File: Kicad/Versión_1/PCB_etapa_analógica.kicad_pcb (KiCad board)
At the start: 2 copper layers, 83 x 63 mm, 44 parts, among them J1 Conn_01x01_Pin, J12 Conn_01x01_Pin, J13 Conn_01x01_Pin, J14 Conn_01x01_Pin, J15 Conn_01x01_Pin, J2 Conn_01x01_Pin, J3 Conn_01x01_Pin, J4 Conn_01x01_Pin, J5 Conn_01x01_Pin, J6 Conn_01x01_Pin, J7 Conn_01x01_Pin, U1 AD620, U2 TL084, U4 TL084, U5 TL082

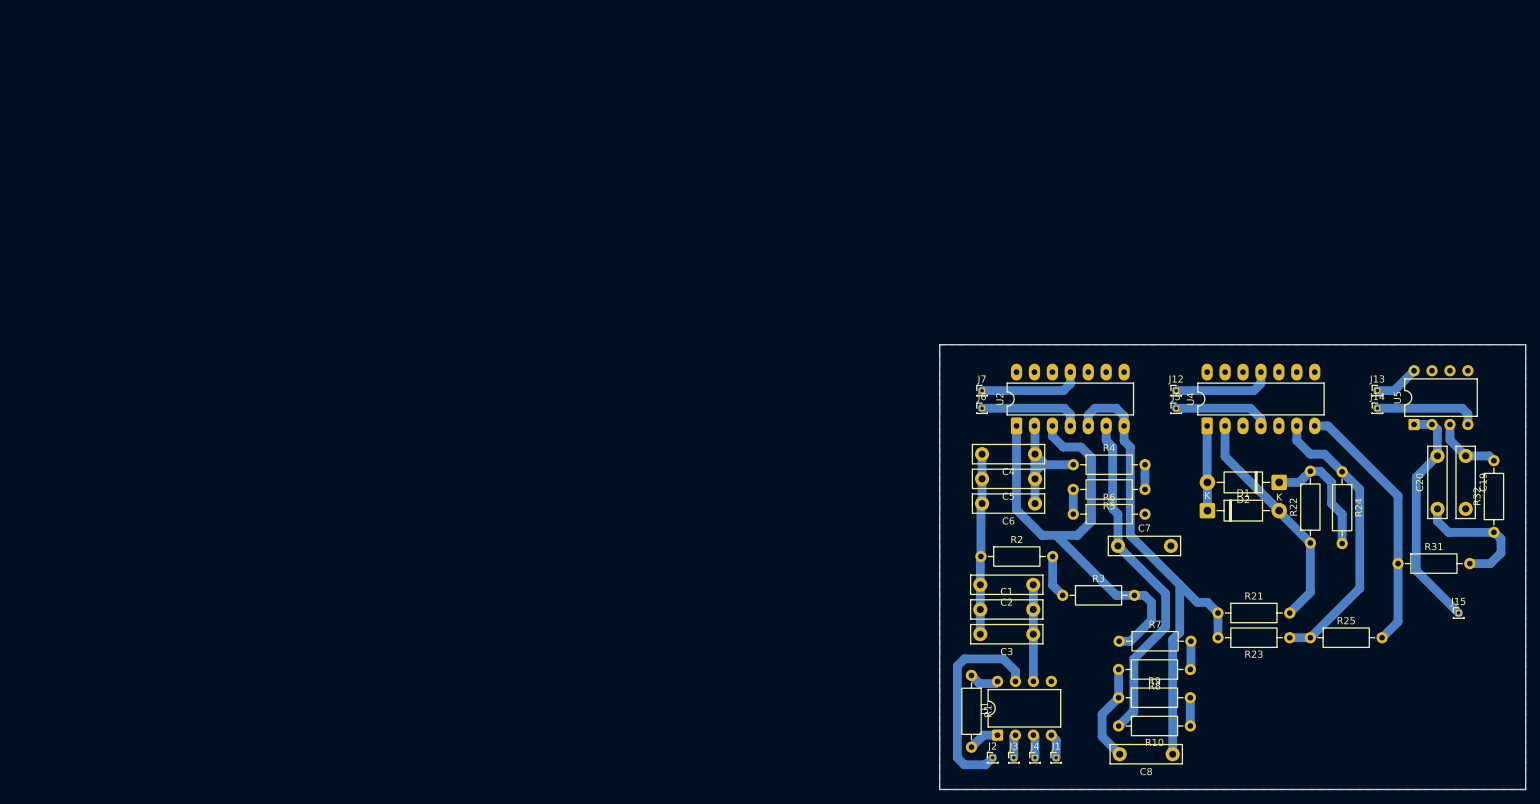
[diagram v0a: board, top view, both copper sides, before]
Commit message: feat(modelos): Añado modelo final de la ortesis
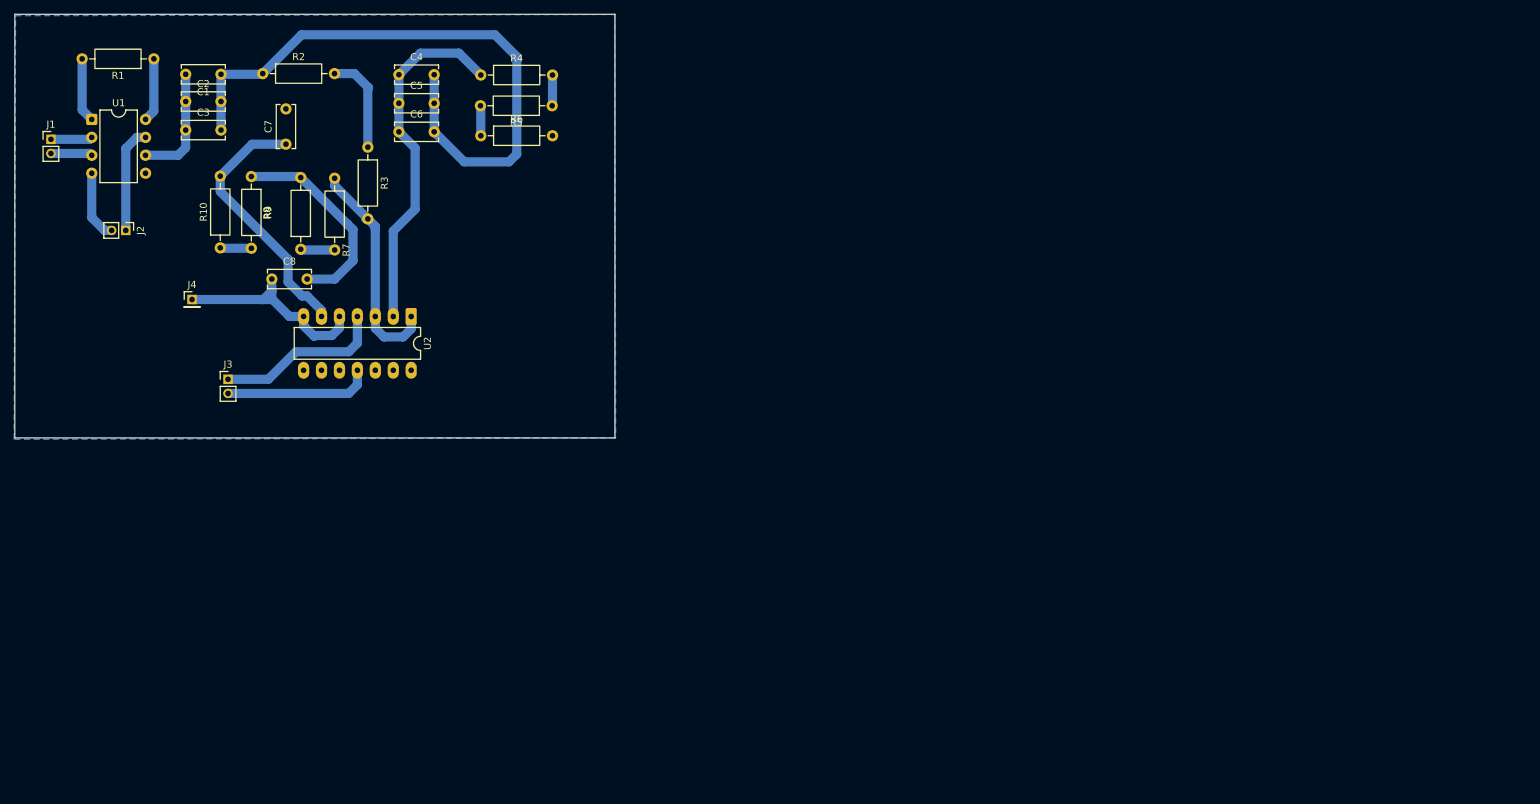
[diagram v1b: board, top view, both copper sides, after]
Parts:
- removed C19, C20: C, Capacitor_THT:C_Rect_L10.0mm_W2.5mm_P7.50mm_MKS4
- removed D1, D2: D, Diode_THT:D_DO-41_SOD81_P10.16mm_Horizontal
- removed J12, J13, J14, J15, J5, J6, J7: Conn_01x01_Pin, Connector_PinHeader_1.00mm:PinHeader_1x01_P1.00mm_Vertical
- removed R21, R22, R23, R24, R25, R31, R32: R, Resistor_THT:R_Axial_DIN0207_L6.3mm_D2.5mm_P10.16mm_Horizontal
- removed U4: TL084, Package_DIP:DIP-14_W7.62mm_LongPads
- removed U5: TL082, Package_DIP:DIP-8_W7.62mm
- C1, C2, C3, C4, C5, C6, C7, C8: footprint Capacitor_THT:C_Rect_L10.0mm_W2.5mm_P7.50mm_MKS4 -> Capacitor_THT:C_Disc_D6.0mm_W2.5mm_P5.00mm
- J1, J2, J3: value Conn_01x01_Pin -> Conn_01x02_Pin; footprint Connector_PinHeader_1.00mm:PinHeader_1x01_P1.00mm_Vertical -> Connector_PinHeader_2.00mm:PinHeader_1x02_P2.00mm_Vertical
- J4: footprint Connector_PinHeader_1.00mm:PinHeader_1x01_P1.00mm_Vertical -> Connector_PinHeader_2.00mm:PinHeader_1x01_P2.00mm_Vertical
- moved J1 167.2 mm to (19.1, 30.9)
- moved U1 155.1 mm to (24.9, 28.1), turned to 0 degrees
- moved R10 153.2 mm to (43.1, 46.3), turned to 90 degrees
- moved R1 145.0 mm to (33.7, 19.5), turned to 180 degrees
- moved C8 144.3 mm to (50.4, 50.7), turned to 0 degrees
- moved J2 143.7 mm to (29.7, 43.8), turned to -90 degrees
- moved R9 143.3 mm to (47.5, 36.2), turned to -90 degrees
- moved C3 139.7 mm to (38.2, 29.6), turned to 0 degrees
- moved R8 139.4 mm to (54.5, 46.5), turned to 90 degrees
- moved C2 138.2 mm to (38.2, 25.6), turned to 0 degrees
- moved J4 135.9 mm to (39.1, 53.6)
- moved C1 131.6 mm to (43.2, 21.7), turned to 180 degrees
- moved C7 130.9 mm to (52.4, 31.6), turned to 90 degrees
- moved R7 129.0 mm to (59.3, 36.4), turned to -90 degrees
- moved J3 123.5 mm to (44.2, 64.9)
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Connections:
- C8 pad 1: Net-(U2B-+) -> Net-(J4-Pin_1)
- U1 pad 2: Net-(J3-Pin_1) -> Net-(J1-Pin_1)
- U1 pad 3: Net-(J4-Pin_1) -> Net-(J1-Pin_2)
- U1 pad 4: Net-(J1-Pin_1) -> Net-(J2-Pin_2)
- U2 pad 11: Net-(J7-Pin_1) -> Net-(J3-Pin_2)
- U2 pad 4: Net-(J6-Pin_1) -> Net-(J3-Pin_1)
- U2 pad 5: Net-(U2B-+) -> Net-(J4-Pin_1)
- U2 pad 7: Net-(U2B-+) -> Net-(J4-Pin_1)
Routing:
- net Net-(U2B-+): track 69.6 -> 0.00 mm
- net Net-(C1-Pad1): track 25.6 -> 89.3 mm
- net Net-(U4B--): track 40.7 -> 0.00 mm
- net Net-(R25-Pad2): track 36.9 -> 0.00 mm
- net Net-(U2A-+): track 67.9 -> 32.1 mm
- net Net-(J15-Pin_1): track 33.3 -> 0.00 mm
- net Net-(D1-A): track 32.7 -> 0.00 mm
- net Net-(U2A--): track 20.0 -> 50.6 mm
- net Net-(J4-Pin_1): track 3.29 -> 30.8 mm
- net Net-(J3-Pin_1): track 3.29 -> 24.2 mm
- net Net-(J3-Pin_2): track 0.00 -> 20.9 mm
- net Net-(C20-Pad1): track 18.8 -> 0.00 mm
- net Net-(D2-K): track 18.0 -> 0.00 mm
- net Net-(C8-Pad2): track 14.0 -> 29.5 mm
- net Net-(J14-Pin_1): track 14.6 -> 0.00 mm
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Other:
- board size 83 x 63 mm -> 85 x 60 mm
